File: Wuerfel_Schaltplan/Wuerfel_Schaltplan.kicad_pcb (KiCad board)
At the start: 2 copper layers, 21 parts, among them SW1 SW_Push, SW2 SW_Push

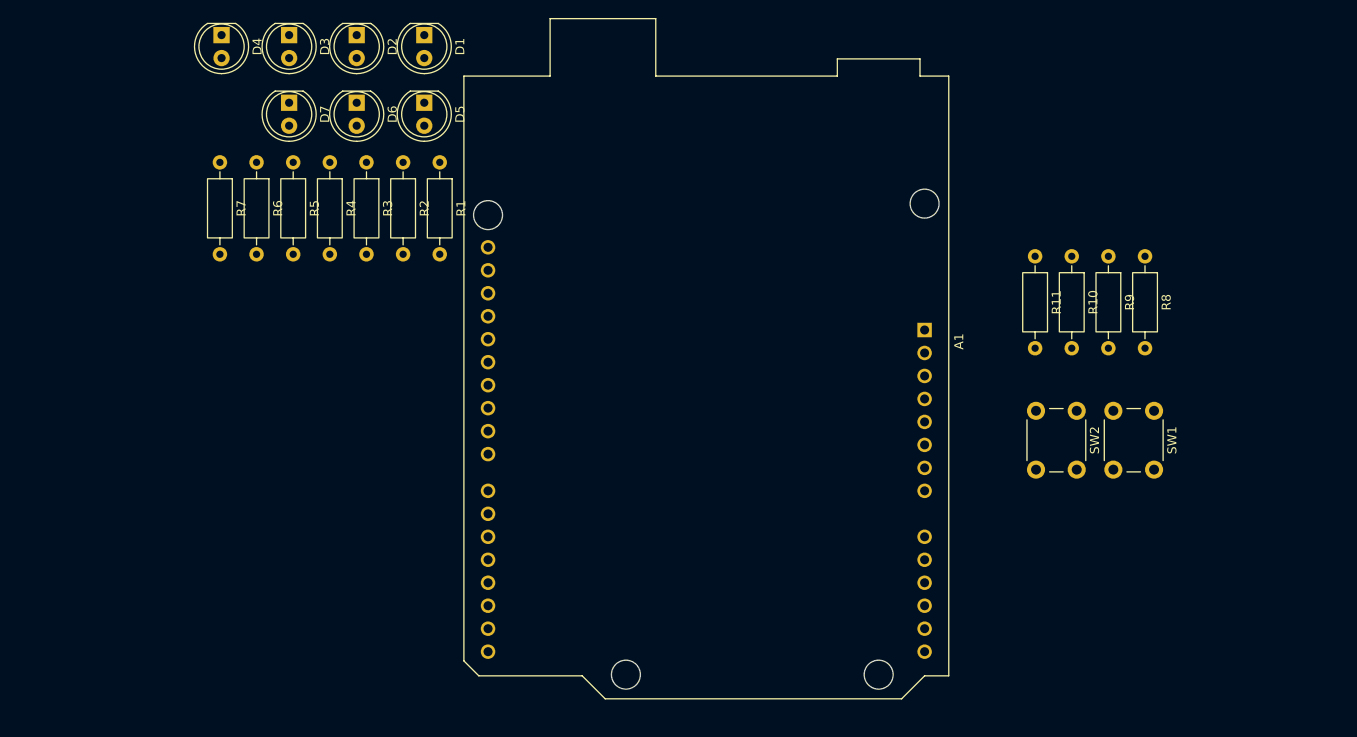
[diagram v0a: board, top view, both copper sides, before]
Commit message: Finish PCB design
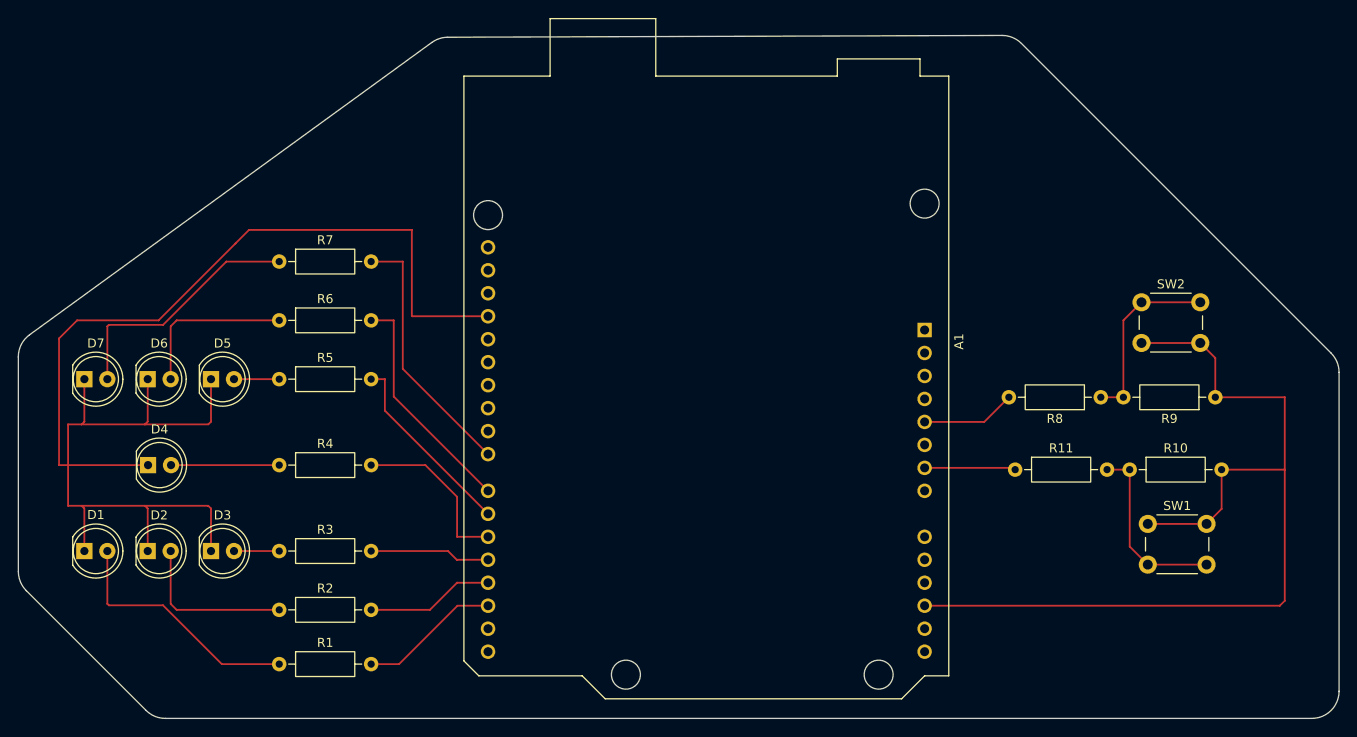
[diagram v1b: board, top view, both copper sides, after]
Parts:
- moved D1 68.3 mm to (97.3, 101.5), turned to 0 degrees
- moved D2 61.5 mm to (104.3, 101.5), turned to 0 degrees
- moved R1 58.2 mm to (118.8, 114.0), turned to 0 degrees
- moved D3 57.7 mm to (111.3, 101.5), turned to 0 degrees
- moved R2 51.3 mm to (118.8, 108.0), turned to 0 degrees
- moved D4 48.2 mm to (104.3, 92.0), turned to 0 degrees
- moved R3 44.0 mm to (118.8, 101.5), turned to 0 degrees
- moved D5 38.6 mm to (111.3, 82.5), turned to 0 degrees
- moved D6 38.3 mm to (104.3, 82.5), turned to 0 degrees
- moved D7 38.0 mm to (97.3, 82.5), turned to 0 degrees
- moved R4 33.9 mm to (118.8, 92.0), turned to 0 degrees
- moved R10 24.4 mm to (212.9, 92.5), turned to 0 degrees
- moved R5 24.0 mm to (118.8, 82.5), turned to 0 degrees
- moved R11 23.7 mm to (200.2, 92.5), turned to 0 degrees
- moved R9 19.6 mm to (222.3, 84.5), turned to 180 degrees
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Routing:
- net Net-(D1-K): track 0.00 -> 156.5 mm
- net Net-(A1-A3): track 0.00 -> 103.6 mm
- net Net-(A1-D8): track 0.00 -> 28.7 mm
- net Net-(D7-A): track 0.00 -> 27.8 mm
- net Net-(D1-A): track 0.00 -> 27.6 mm
- net Net-(A1-D7): track 0.00 -> 25.7 mm
- net Net-(A1-D6): track 0.00 -> 21.1 mm
- net Net-(R8-Pad1): track 0.00 -> 20.3 mm
- net Net-(R10-Pad1): track 0.00 -> 20.3 mm
- net Net-(A1-D5): track 0.00 -> 18.8 mm
- net Net-(D6-A): track 0.00 -> 18.1 mm
- net Net-(D2-A): track 0.00 -> 18.1 mm
- net Net-(A1-D2): track 0.00 -> 15.6 mm
- net Net-(A1-D3): track 0.00 -> 14.2 mm
- net Net-(A1-D4): track 0.00 -> 13.4 mm
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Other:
- board outline added: 146 x 75.5 mm
